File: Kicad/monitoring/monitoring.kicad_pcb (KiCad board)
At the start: 2 copper layers, 98.7 x 51.1 mm, 19 parts, among them J1 Module1, J2 Module2, J3 Module3, J4 buttons, J5 Display, J6 Display, J7 DC_in_outout, U1 4052, U3 L7805, U4 L7805

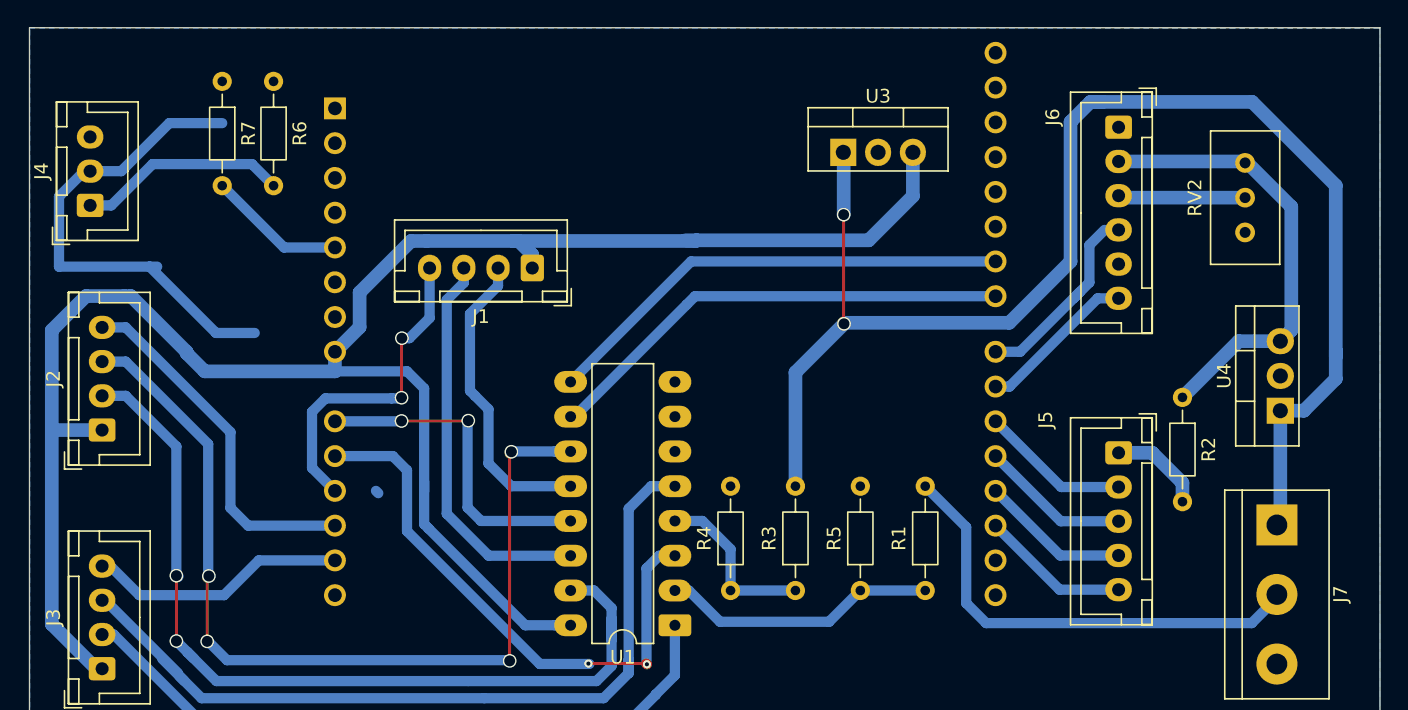
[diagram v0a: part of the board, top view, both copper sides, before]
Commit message: Update #auto_saved_files#, Arduino_UNO_R2.kicad_mod, fp-info-cache, and 9 more files
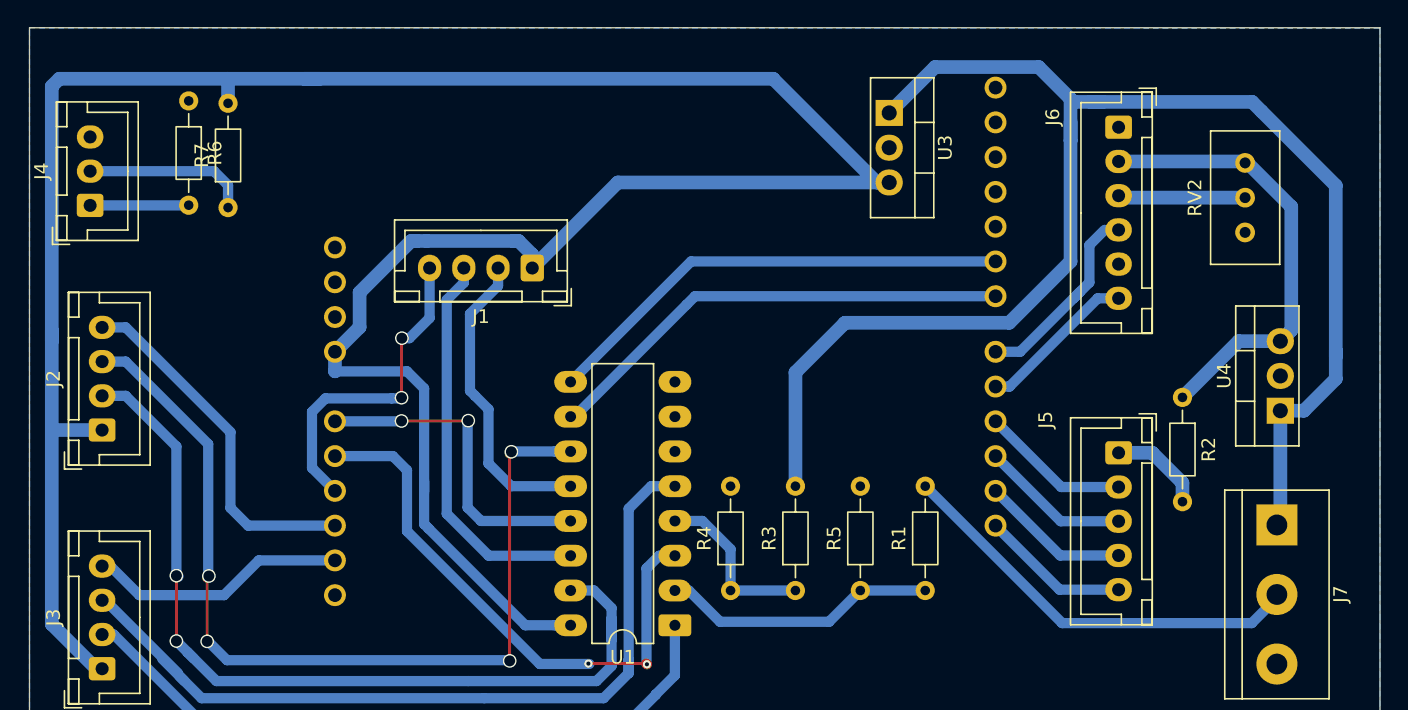
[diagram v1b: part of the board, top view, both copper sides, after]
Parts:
- A1: footprint Module:Arduino_UNO_R2 -> custom_lib:Arduino_UNO_R2
- moved R7 9.23 mm to (75.0, 66.3), turned to 90 degrees
- moved R6 6.36 mm to (72.2, 58.5)
- moved U3 4.42 mm to (123.3, 59.3), turned to -90 degrees
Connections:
- A1 pad 5: Net-(A1-+5V) -> unconnected-(A1-+5V-Pad5)
- R7 pad 2: Net-(A1-+5V) -> +5VA
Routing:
- net +5VA: track 144.5 -> 200.6 mm
- net /COMMON: track 36.1 -> 12.6 mm
- net Net-(A1-+5V): track 10.1 -> 0.00 mm
- net /UP: track 15.4 -> 7.26 mm
- net VCC: track 105.8 -> 111.4 mm, vias 2 -> 0
- net /ps_out: track 34.5 -> 31.3 mm

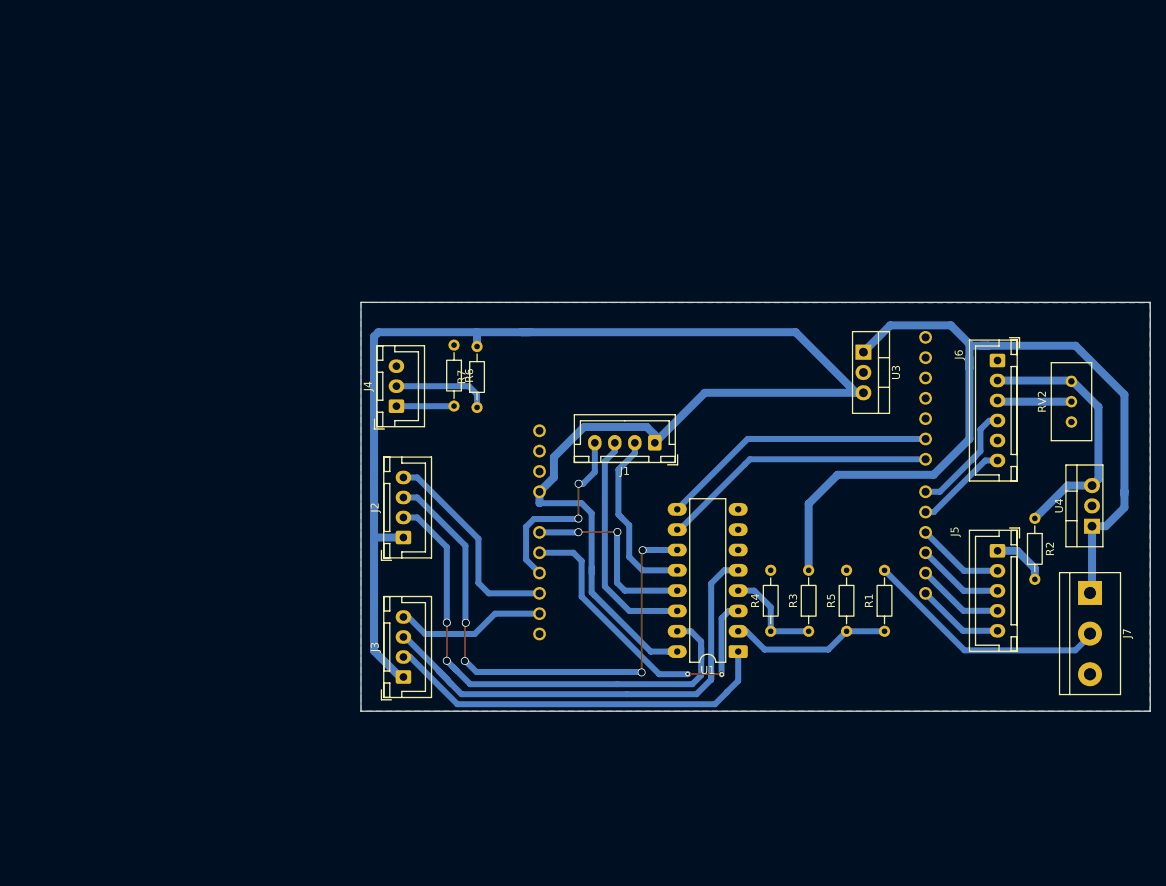
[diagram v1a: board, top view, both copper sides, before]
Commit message: Ready for 1st test
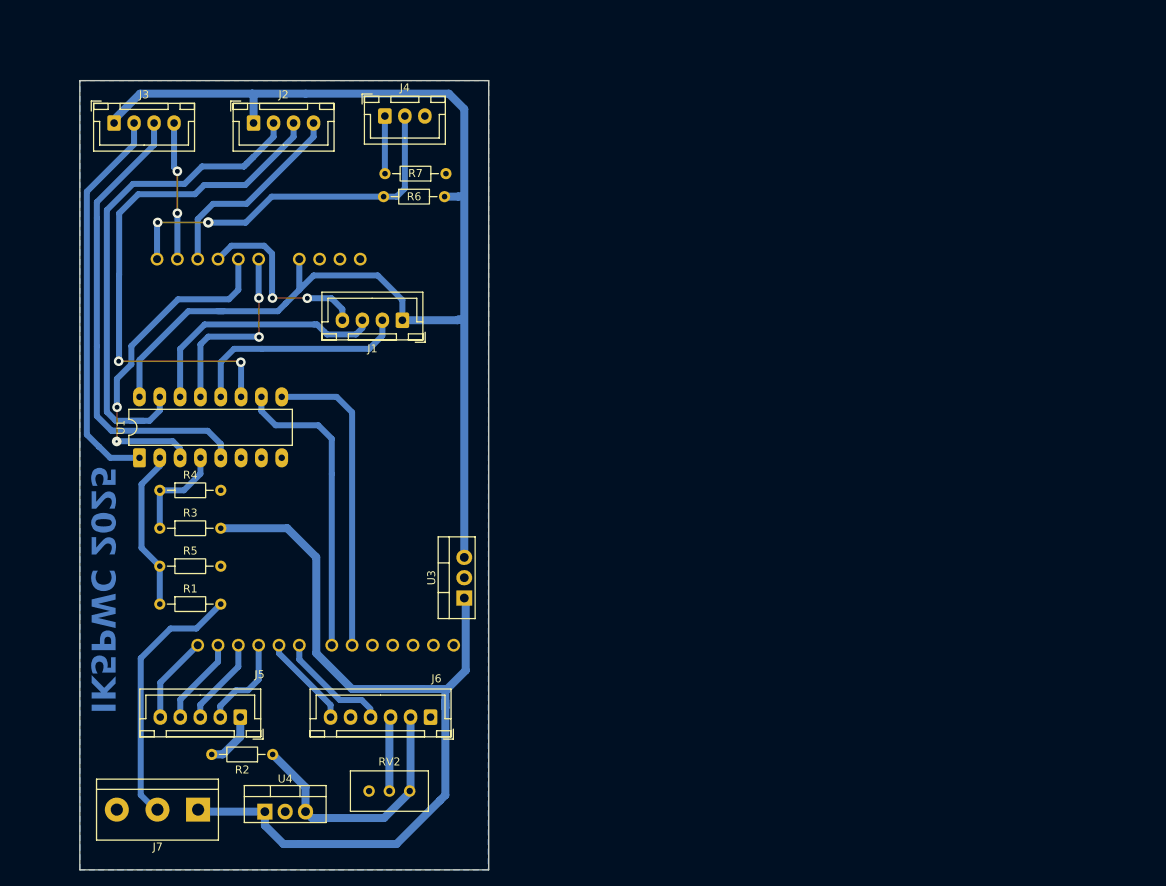
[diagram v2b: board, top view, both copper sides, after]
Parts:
- moved J7 114.7 mm to (40.2, 116.5), turned to 180 degrees
- moved U4 109.4 mm to (48.5, 116.8), turned to 0 degrees
- moved R2 99.7 mm to (49.5, 109.6), turned to 180 degrees
- moved RV2 97.3 mm to (66.6, 114.2), turned to 0 degrees
- moved J5 96.9 mm to (45.5, 105.0), turned to 180 degrees
- moved R1 90.7 mm to (35.4, 90.8), turned to 0 degrees
- moved R5 86.2 mm to (35.4, 86.1), turned to 0 degrees
- moved J6 83.7 mm to (69.2, 105.0), turned to 180 degrees
- moved R3 82.1 mm to (35.4, 81.4), turned to 0 degrees
- moved U1 78.7 mm to (32.9, 72.6), turned to 90 degrees
- moved R4 78.4 mm to (35.4, 76.6), turned to 0 degrees
- moved J3 78.1 mm to (29.7, 30.7), turned to 0 degrees
- moved U3 58.6 mm to (73.5, 90.1), turned to 90 degrees
- moved J2 55.1 mm to (47.1, 30.7), turned to 0 degrees
- moved J4 36.3 mm to (63.5, 29.8), turned to 0 degrees
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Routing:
- net +5VA: track 200.6 -> 165.4 mm
- net /COMMON: track 12.6 -> 46.7 mm, vias 0 -> 2
- net /m1_Iout: track 22.4 -> 27.8 mm
- net VCC: track 111.4 -> 106.3 mm
- net /BCD-2: track 34.7 -> 38.7 mm
- net /BCD-1: track 34.7 -> 37.8 mm
- net /m1_Ibat: track 28.8 -> 31.9 mm
- net /m3_Ibat: track 61.4 -> 59.5 mm
- net /ps_out: track 31.3 -> 33.2 mm
- net /m2_Ibat: track 68.3 -> 66.9 mm, vias 4 -> 2
- net /m3_Vbat: track 18.9 -> 17.8 mm, vias 0 -> 2
- net Net-(A1-A1): track 41.0 -> 42.0 mm
- net /LCD_D7: track 11.0 -> 11.9 mm
- net /m2_Vbat: track 26.3 -> 25.5 mm
- net /m2_Iout: track 65.1 -> 64.4 mm, vias 2 -> 0
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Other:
- board size 98.7 x 51.1 mm -> 51.1 x 98.7 mm
- board text added: "IK5PWC 2025"

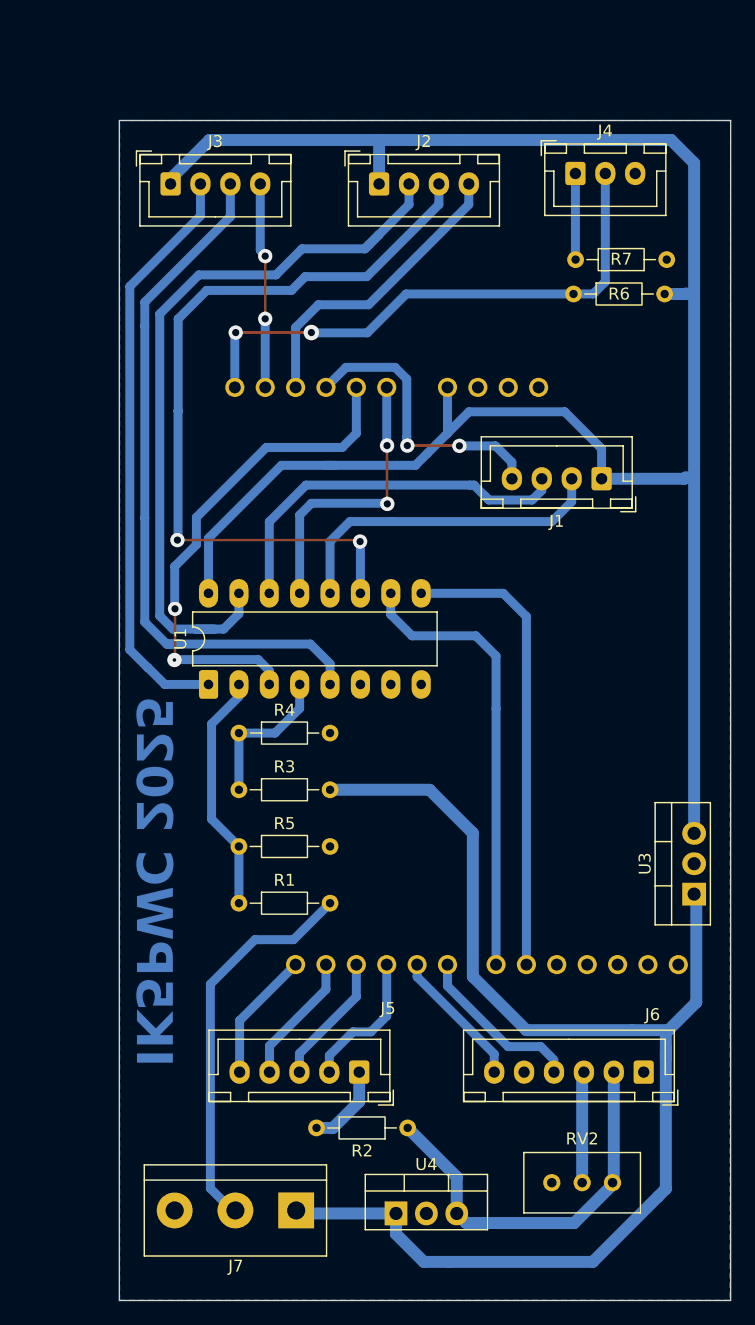
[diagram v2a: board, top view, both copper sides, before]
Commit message: Update .cproject, .project, UPSMonitor.ino, and 29 more files
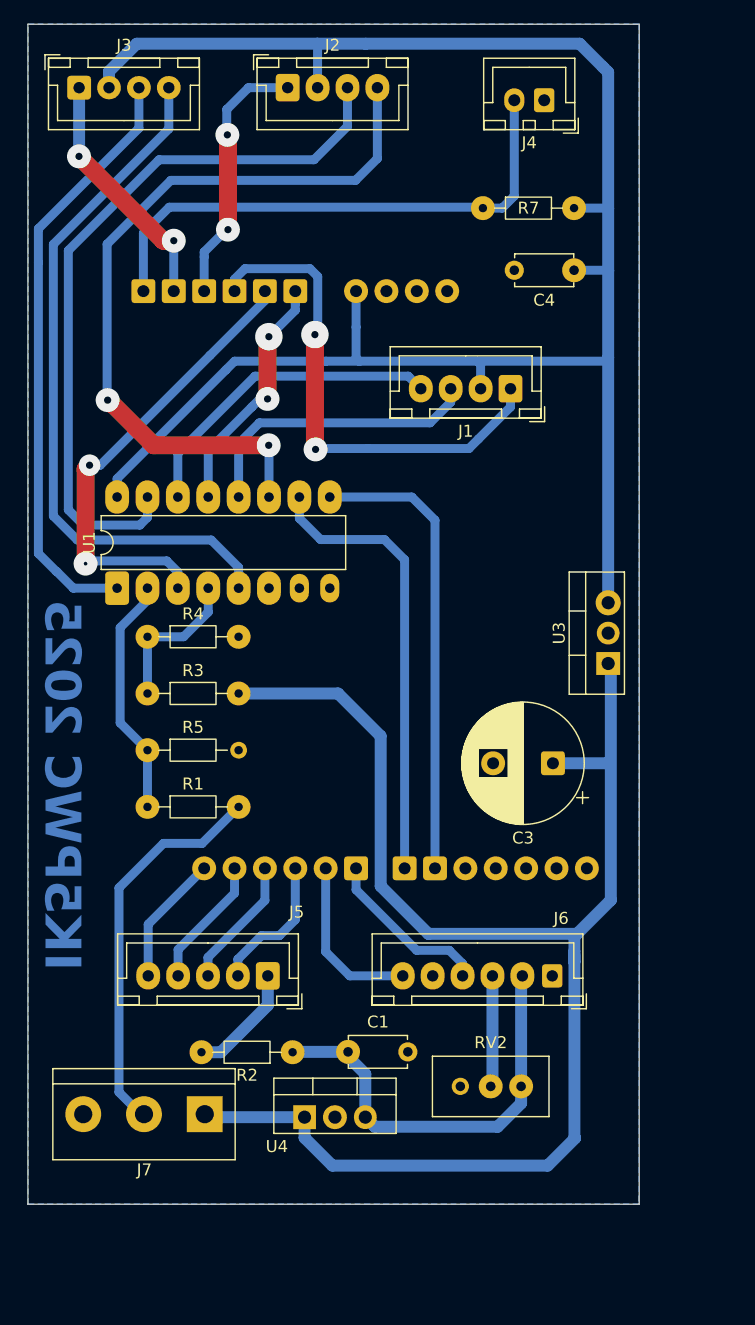
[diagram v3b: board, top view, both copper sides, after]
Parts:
- removed R6: 10K, Resistor_THT:R_Axial_DIN0204_L3.6mm_D1.6mm_P7.62mm_Horizontal
- added C1: 100 nF, Capacitor_THT:C_Disc_D4.7mm_W2.5mm_P5.00mm, F.Cu at (44.5, 103.3)
- added C3: 220 uF, Capacitor_THT:CP_Radial_D10.0mm_P5.00mm, F.Cu at (61.6, 79.1)
- added C4: 100 nF, Capacitor_THT:C_Disc_D4.7mm_W2.5mm_P5.00mm, F.Cu at (63.4, 37.9)
- J4: footprint Connector_JST:JST_XH_B3B-XH-A_1x03_P2.50mm_Vertical -> Connector_JST:JST_XH_B2B-XH-A_1x02_P2.50mm_Vertical
- moved U3 20.6 mm to (66.3, 70.8)
- moved R2 11.5 mm to (39.9, 103.3)
- moved R3 11.1 mm to (27.8, 73.3)
- moved A1 11.1 mm to (63.0, 39.7)
- moved J2 11.1 mm to (39.5, 22.7)
- moved J7 11.1 mm to (32.5, 108.5)
- moved RV2 11.1 mm to (59.0, 106.2)
- moved U1 11.1 mm to (25.2, 64.5)
- moved U4 11.1 mm to (40.9, 108.7)
- moved J3 11.1 mm to (22.0, 22.7)
- moved R1 11.1 mm to (27.8, 82.8)
- moved R4 11.1 mm to (27.8, 68.6)
- moved R5 11.1 mm to (27.8, 78.0)
- moved J5 11.1 mm to (37.8, 96.9)
- moved J6 11.1 mm to (61.6, 96.9)
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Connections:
- net /COMMON renamed /PUSH
- net /dc_Vin renamed /ps_Vin
- J1 pad 1: +5VA -> /m1_Vbat
- J1 pad 2: /m1_Iout -> +5VA
- J1 pad 3: /m1_Ibat -> /m1_Iout
- J1 pad 4: /m1_Vbat -> /m1_Ibat
- J2 pad 1: +5VA -> /m2_Vbat
- J2 pad 2: /m2_Iout -> +5VA
- J2 pad 3: /m2_Ibat -> /m2_Iout
- J2 pad 4: /m2_Vbat -> /m2_Ibat
- J3 pad 1: +5VA -> /m3_Vbat
- J3 pad 2: /m3_Iout -> +5VA
- J3 pad 3: /m3_Ibat -> /m3_Iout
- J3 pad 4: /m3_Vbat -> /m3_Ibat
- J4 pad 1: /UP -> GND
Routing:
- net /m1_Vbat: track 24.2 -> 43.1 mm
- net VCC: track 106.3 -> 125.2 mm
- net +5VA: track 165.4 -> 154.0 mm
- net /UP: track 7.26 -> 0.00 mm
- net /m1_Ibat: track 31.9 -> 27.1 mm
- net /m2_Vbat: track 25.5 -> 22.0 mm, vias 0 -> 2
- net Net-(A1-A0): track 24.0 -> 20.8 mm
- net /m1_Iout: track 27.8 -> 24.8 mm
- net /m3_Vbat: track 17.8 -> 20.8 mm
- net +5VD: track 33.0 -> 35.7 mm
- net /LCD_EN: track 11.7 -> 14.3 mm
- net /m2_Iout: track 64.4 -> 61.9 mm
- net Net-(A1-A1): track 42.0 -> 39.6 mm
- net /m2_Ibat: track 66.9 -> 64.6 mm
- net /PUSH: track 46.7 -> 45.1 mm, vias 2 -> 0
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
